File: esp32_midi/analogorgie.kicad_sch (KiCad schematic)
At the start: 64 parts, among them U10 BL1551, U108 BL1551, U11 BL1551, U114 BL1551, U12 BL1551, U13 BL1551, U14 BL1551, U15 BL1551, U16 BL1551, U17 BL1551, U18 BL1551, U19 BL1551, U20 BL1551, U21 BL1551, U22 BL1551, U23 BL1551, U24 BL1551, U25 BL1551, U26 BL1551, U27 BL1551, U28 BL1551, U29 BL1551, U30 BL1551, U31 BL1551, U32 BL1551, U33 BL1551, U34 BL1551, U35 BL1551, U6 BL1551, U7 BL1551, U8 BL1551, U9 BL1551

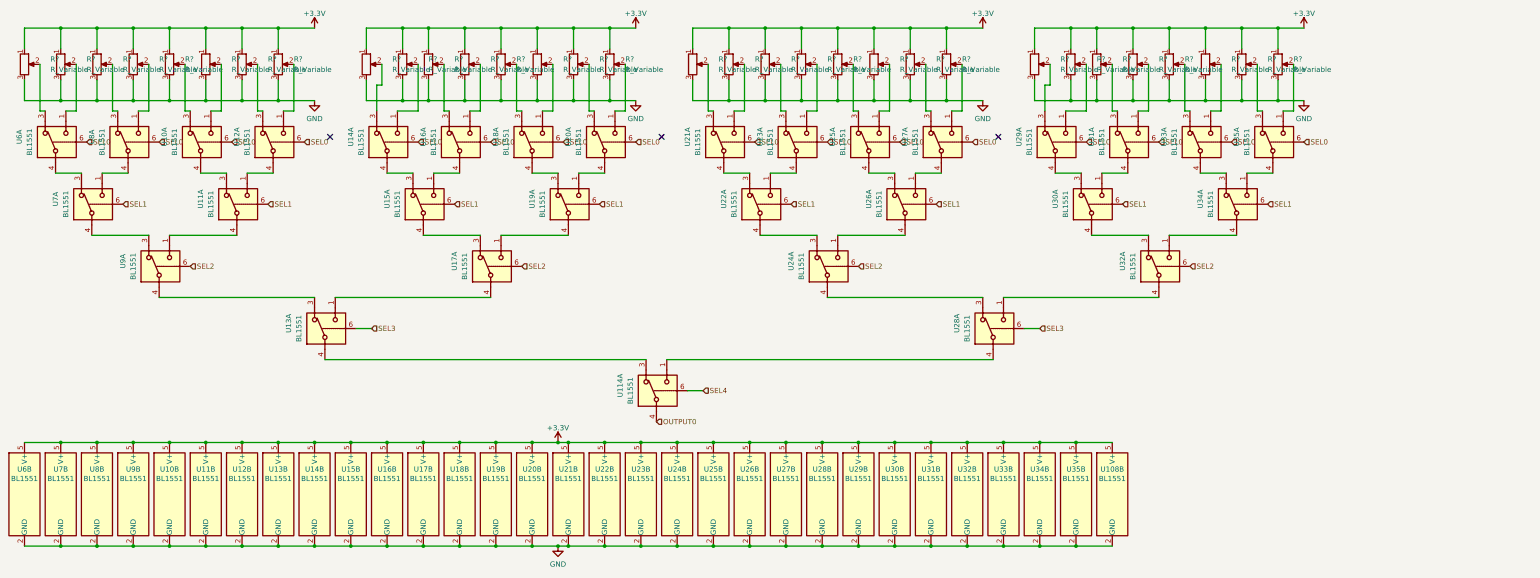
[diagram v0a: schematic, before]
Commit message: muchos viasos
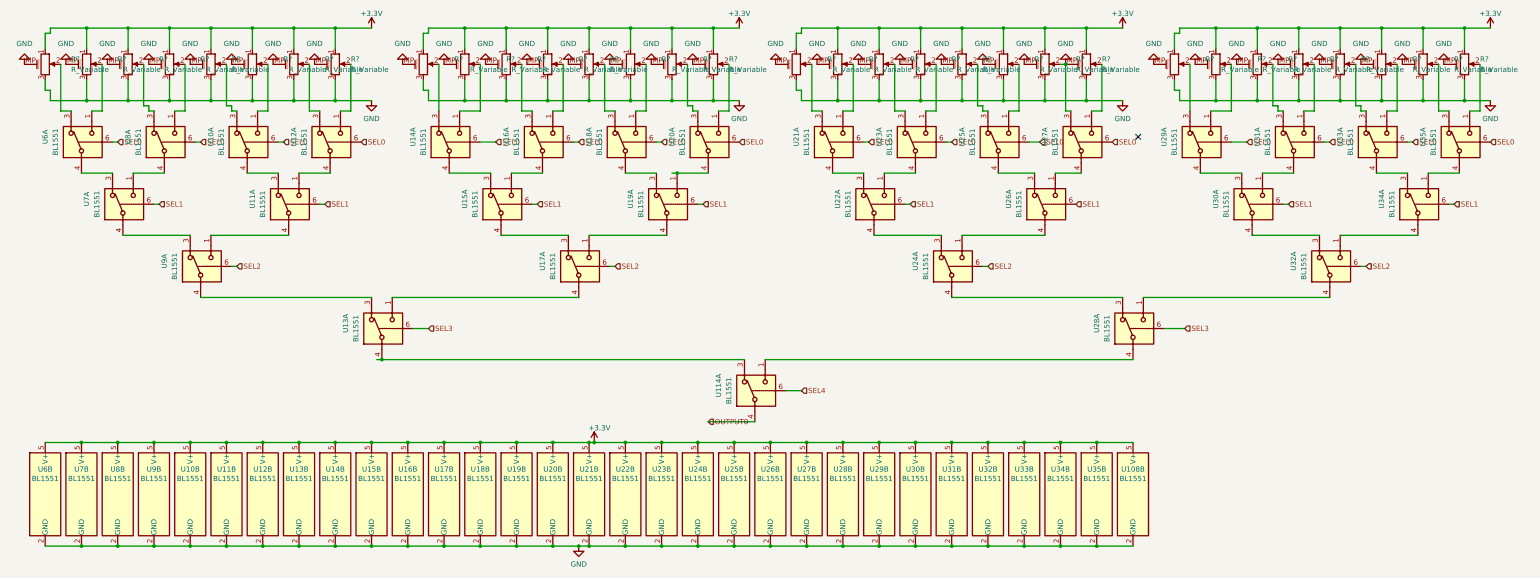
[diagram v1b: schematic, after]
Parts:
- R? (x32): symbol Device:R_Potentiometer -> Device:R_Potentiometer_MountingPin
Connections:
- net GND: now also R?.2, R?.MP (MountPin), R?.MP (MountPin), R?.MP (MountPin), R?.MP (MountPin), R?.MP (MountPin), R?.MP (MountPin), R?.MP (MountPin), R?.MP (MountPin), R?.MP (MountPin), R?.MP (MountPin), R?.MP (MountPin), R?.MP (MountPin), R?.MP (MountPin), R?.MP (MountPin), R?.MP (MountPin), R?.MP (MountPin), R?.MP (MountPin), R?.MP (MountPin), R?.MP (MountPin), R?.MP (MountPin), R?.MP (MountPin), R?.MP (MountPin), R?.MP (MountPin), R?.MP (MountPin), R?.MP (MountPin), R?.MP (MountPin), R?.MP (MountPin), R?.MP (MountPin), R?.MP (MountPin), R?.MP (MountPin), R?.MP (MountPin), R?.MP (MountPin), U27.3
- no-connect marks 3 -> 1
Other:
- moved on the sheet: U108B, U10A, U10B, U114A, U11A, U11B, U12A, U12B, U13A, U13B, U14A, U14B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

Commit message: Everything changed
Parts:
- R? (x24): footprint ordentliche-teile:Potentiometer_vom_markt -> Potentiometer_THT:Potentiometer_Alps_RK09L_Single_Vertical
